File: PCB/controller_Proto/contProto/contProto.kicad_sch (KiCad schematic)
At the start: 71 parts, among them J1 Conn_01x05, J10 JST_1mm_3, J11 JST_1mm_3, J12 JST_1mm_3, J13 Conn_01x02_Socket, J14 Conn_01x02_Socket, J15 Conn_01x04, J16 Conn_01x04, J17 Conn_01x10_Pin, J18 JST_1mm_3, J19 Conn_01x08_Socket, J2 Conn_01x04, J20 JST_1mm_3, J21 JST_1mm_3, J22 JST_1mm_3, J23 JST_1mm_3, J3 Conn_01x10_Pin, J4 JST_1mm_3, J5 Conn_01x05, J6 JST_1mm_3, J7 Conn_01x05, J8 Conn_01x05, J9 Conn_01x04, SW1 SMD_12x12mm_h8.5mm, SW10 SMD_12x12mm_h8.5mm, SW11 SMD_12x12mm_h8.5mm, SW12 SMD_12x12mm_h8.5mm, SW13 SMD_12x12mm_h8.5mm, SW14 SMD_12x12mm_h8.5mm, SW15 SMD_12x12mm_h8.5mm, SW16 SMD_12x12mm_h8.5mm, SW17 SMD_12x12mm_h8.5mm, SW18 SMD_12x12mm_h8.5mm, SW19 SMD_12x12mm_h8.5mm, SW2 SMD_12x12mm_h8.5mm, SW20 SMD_12x12mm_h8.5mm, SW3 SMD_12x12mm_h8.5mm, SW4 SMD_12x12mm_h8.5mm, SW5 SMD_12x12mm_h8.5mm, SW6 SMD_12x12mm_h8.5mm, SW7 SMD_12x12mm_h8.5mm, SW8 SMD_12x12mm_h8.5mm, SW9 SMD_12x12mm_h8.5mm, U1 ProMicroC, U2 ProMicroC, U3 DRV5033FAxLPG, U4 DRV5033FAxLPG

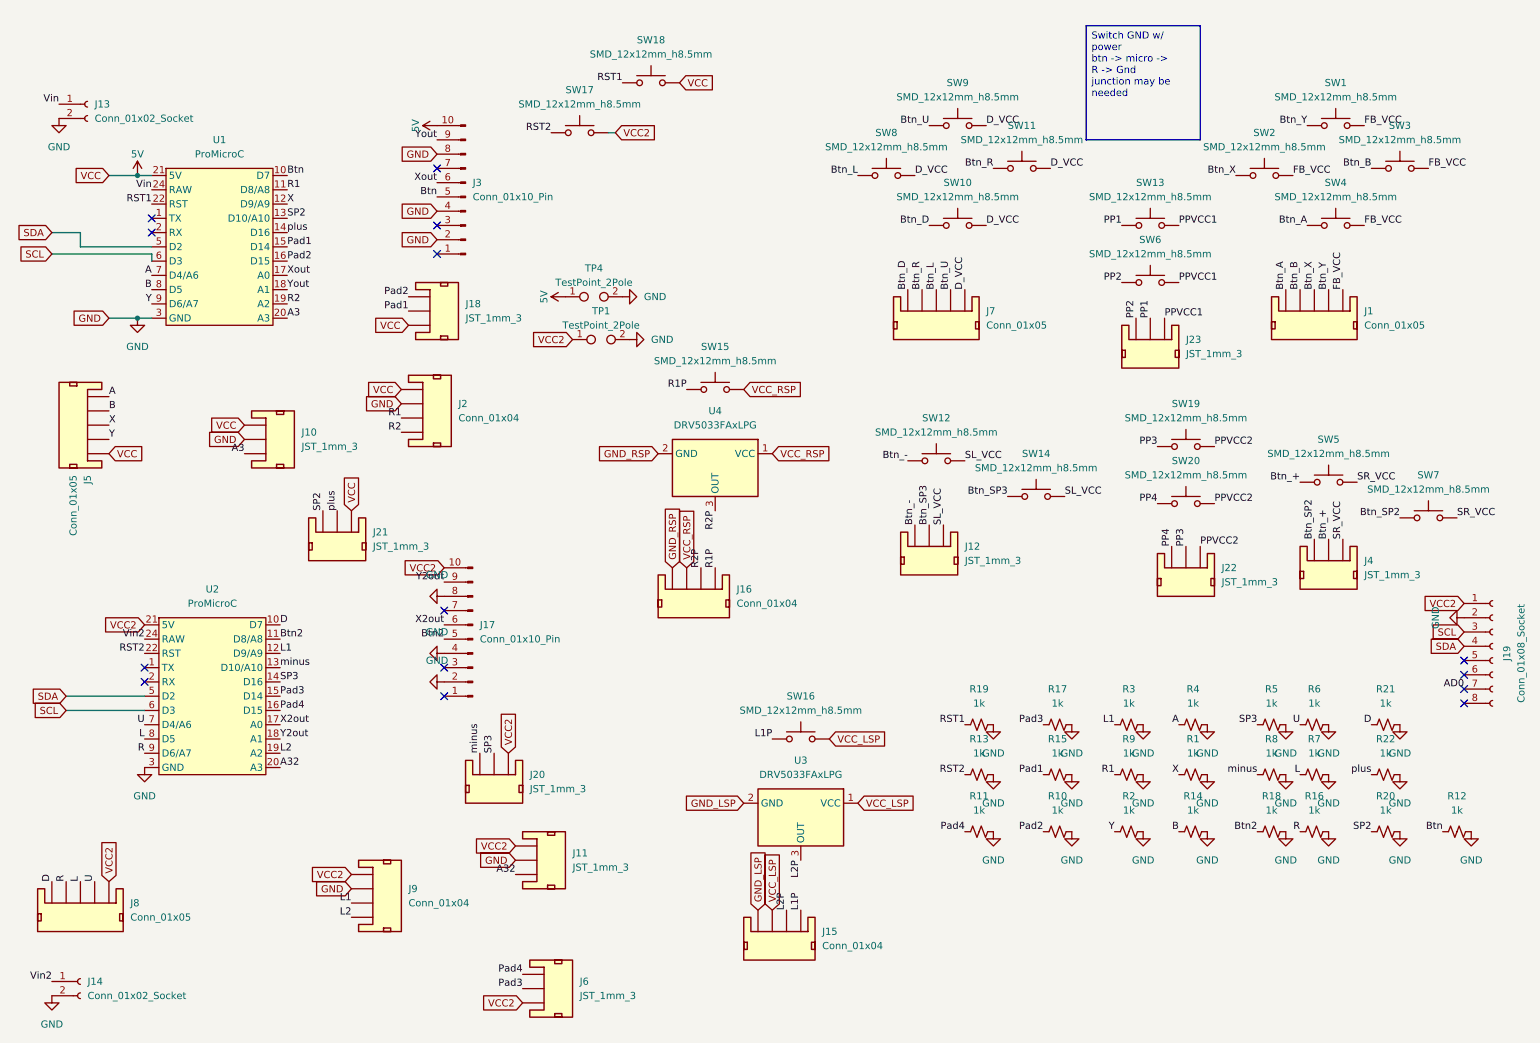
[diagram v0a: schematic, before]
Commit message: finnish shoulder borads
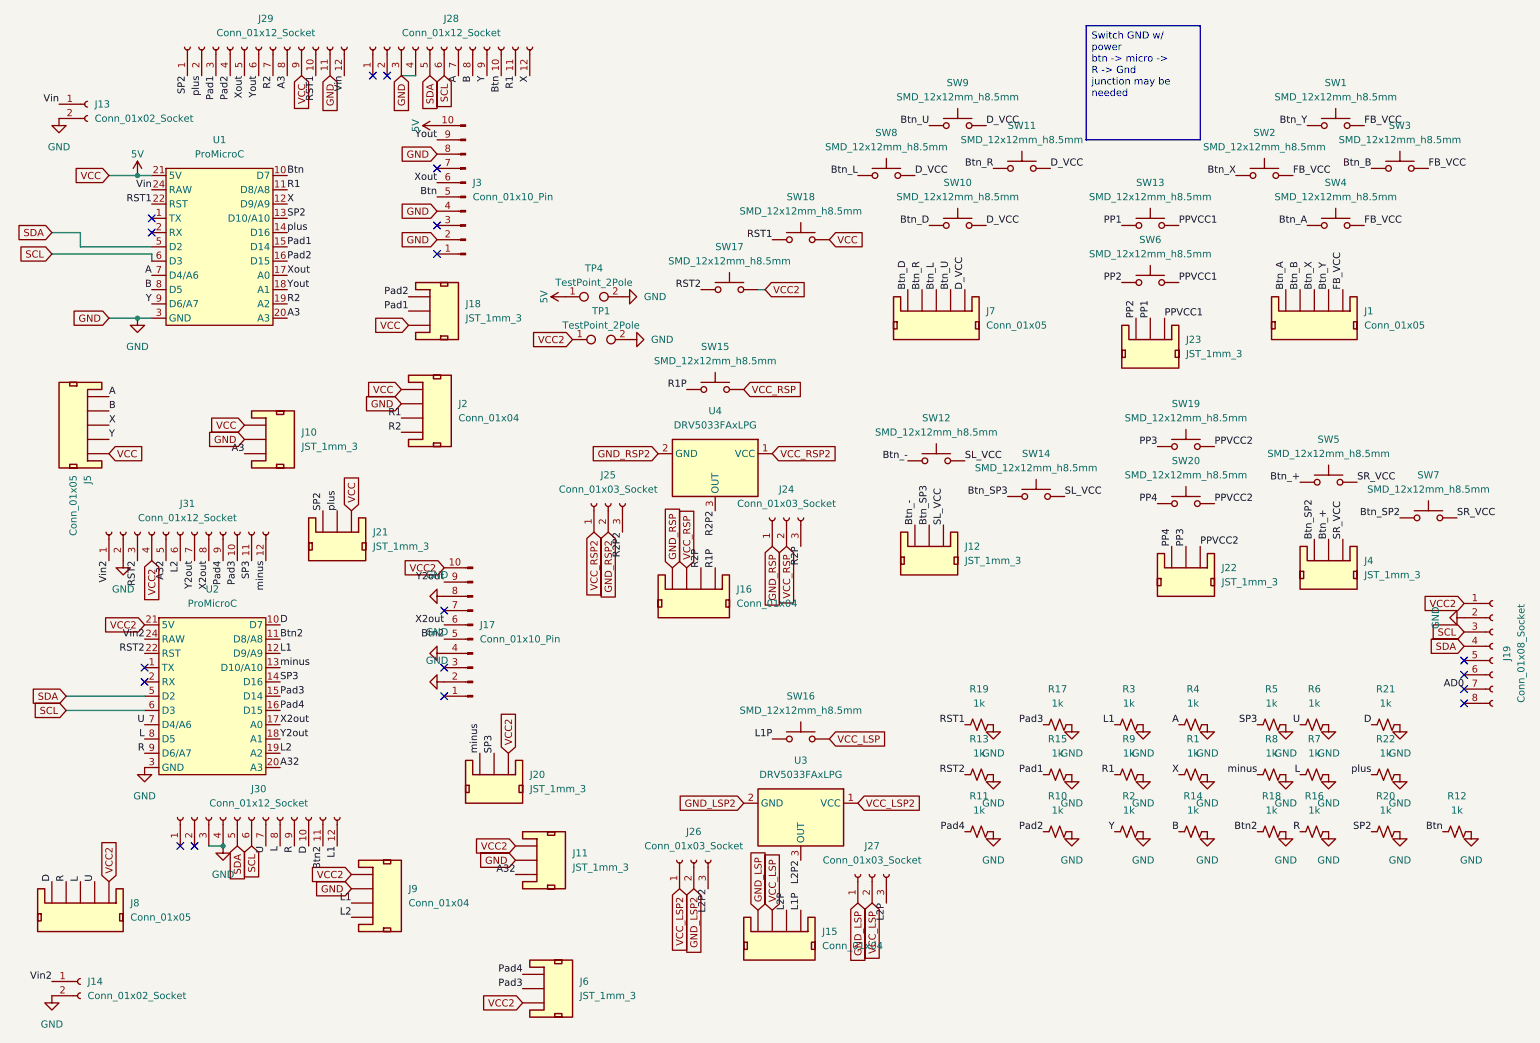
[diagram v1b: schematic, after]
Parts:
- added J24, J25, J26, J27: Conn_01x03_Socket, Connector_PinSocket_2.54mm:PinSocket_1x03_P2.54mm_Vertical, symbol Connector:Conn_01x03_Socket
- added J28, J29, J30, J31: Conn_01x12_Socket, Connector_PinSocket_2.54mm:PinSocket_1x12_P2.54mm_Vertical, symbol Connector:Conn_01x12_Socket
- J19: footprint Connector_PinSocket_1.00mm:PinSocket_1x08_P1.00mm_Vertical -> Connector_PinSocket_2.54mm:PinSocket_1x08_P2.54mm_Vertical
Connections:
- net 5V: now also J29.9 (Pin_9)
- net A: now also J28.7 (Pin_7)
- net A3: now also J29.8 (Pin_8)
- net A32: now also J31.5 (Pin_5)
- net B: now also J28.8 (Pin_8)
- net Btn: now also J28.10 (Pin_10)
- net Btn2: now also J30.11 (Pin_11)
- net D: now also J30.10 (Pin_10)
- net GND: now also J28.3 (Pin_3), J28.4 (Pin_4), J29.11 (Pin_11), J30.3 (Pin_3), J30.4 (Pin_4), J31.2 (Pin_2)
- net GND_LSP: now also J27.1 (Pin_1); no longer U3.2 (GND)
- net GND_RSP: now also J24.1 (Pin_1); no longer U4.2 (GND)
- net L: now also J30.8 (Pin_8)
- net L1: now also J30.12 (Pin_12)
- net L2: now also J31.6 (Pin_6)
- net L2P: now also J27.3 (Pin_3); no longer U3.3 (OUT)
- net Pad1: now also J29.3 (Pin_3)
- net Pad2: now also J29.4 (Pin_4)
- net Pad3: now also J31.10 (Pin_10)
- net Pad4: now also J31.9 (Pin_9)
- net R: now also J30.9 (Pin_9)
- net R1: now also J28.11 (Pin_11)
- net R2: now also J29.7 (Pin_7)
- net R2P: now also J24.3 (Pin_3); no longer U4.3 (OUT)
- net RST1: now also J29.10 (Pin_10)
- net RST2: now also J31.3 (Pin_3)
- net SCL: now also J28.6 (Pin_6), J30.6 (Pin_6)
- net SDA: now also J28.5 (Pin_5), J30.5 (Pin_5)
- net SP2: now also J29.1 (Pin_1)
- net SP3: now also J31.11 (Pin_11)
- net U: now also J30.7 (Pin_7)
- net VCC2: now also J31.4 (Pin_4)
- net VCC_LSP: now also J27.2 (Pin_2); no longer U3.1 (VCC)
- net VCC_RSP: now also J24.2 (Pin_2); no longer U4.1 (VCC)
- net Vin: now also J29.12 (Pin_12)
- net Vin2: now also J31.1 (Pin_1)
- net X: now also J28.12 (Pin_12)
- net X2out: now also J31.8 (Pin_8)
- net Xout: now also J29.5 (Pin_5)
- net Y: now also J28.9 (Pin_9)
- net Y2out: now also J31.7 (Pin_7)
- net Yout: now also J29.6 (Pin_6)
- net minus: now also J31.12 (Pin_12)
- net plus: now also J29.2 (Pin_2)
- new net GND_LSP2: J26.2 (Pin_2), U3.2 (GND)
- new net GND_RSP2: J25.2 (Pin_2), U4.2 (GND)
- new net L2P2: J26.3 (Pin_3), U3.3 (OUT)
- new net R2P2: J25.3 (Pin_3), U4.3 (OUT)
- new net VCC_LSP2: J26.1 (Pin_1), U3.1 (VCC)
- new net VCC_RSP2: J25.1 (Pin_1), U4.1 (VCC)
- no-connect marks 14 -> 18
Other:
- moved on the sheet: SW17, SW18
